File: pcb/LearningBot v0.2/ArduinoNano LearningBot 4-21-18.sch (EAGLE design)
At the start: 22 parts

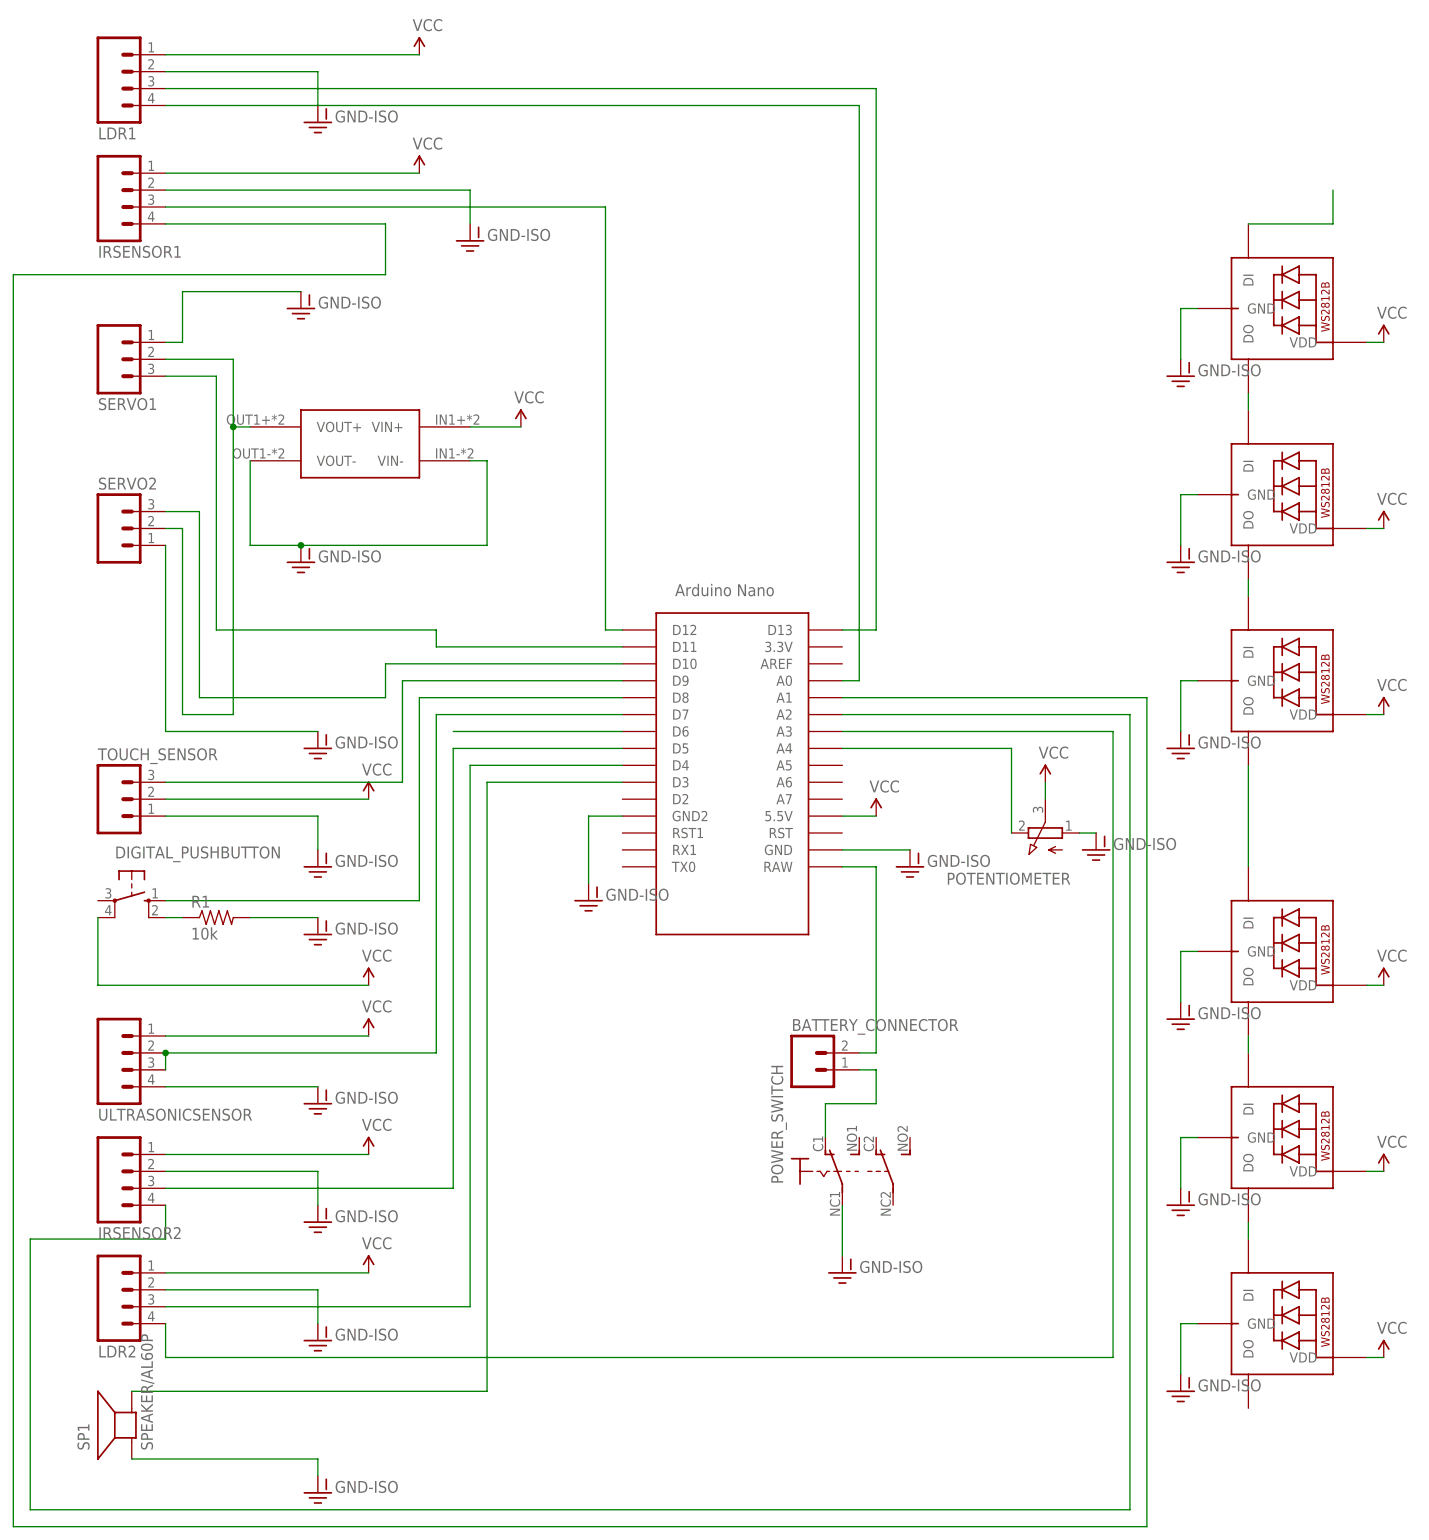
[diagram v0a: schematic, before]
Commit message: Ready for inspection
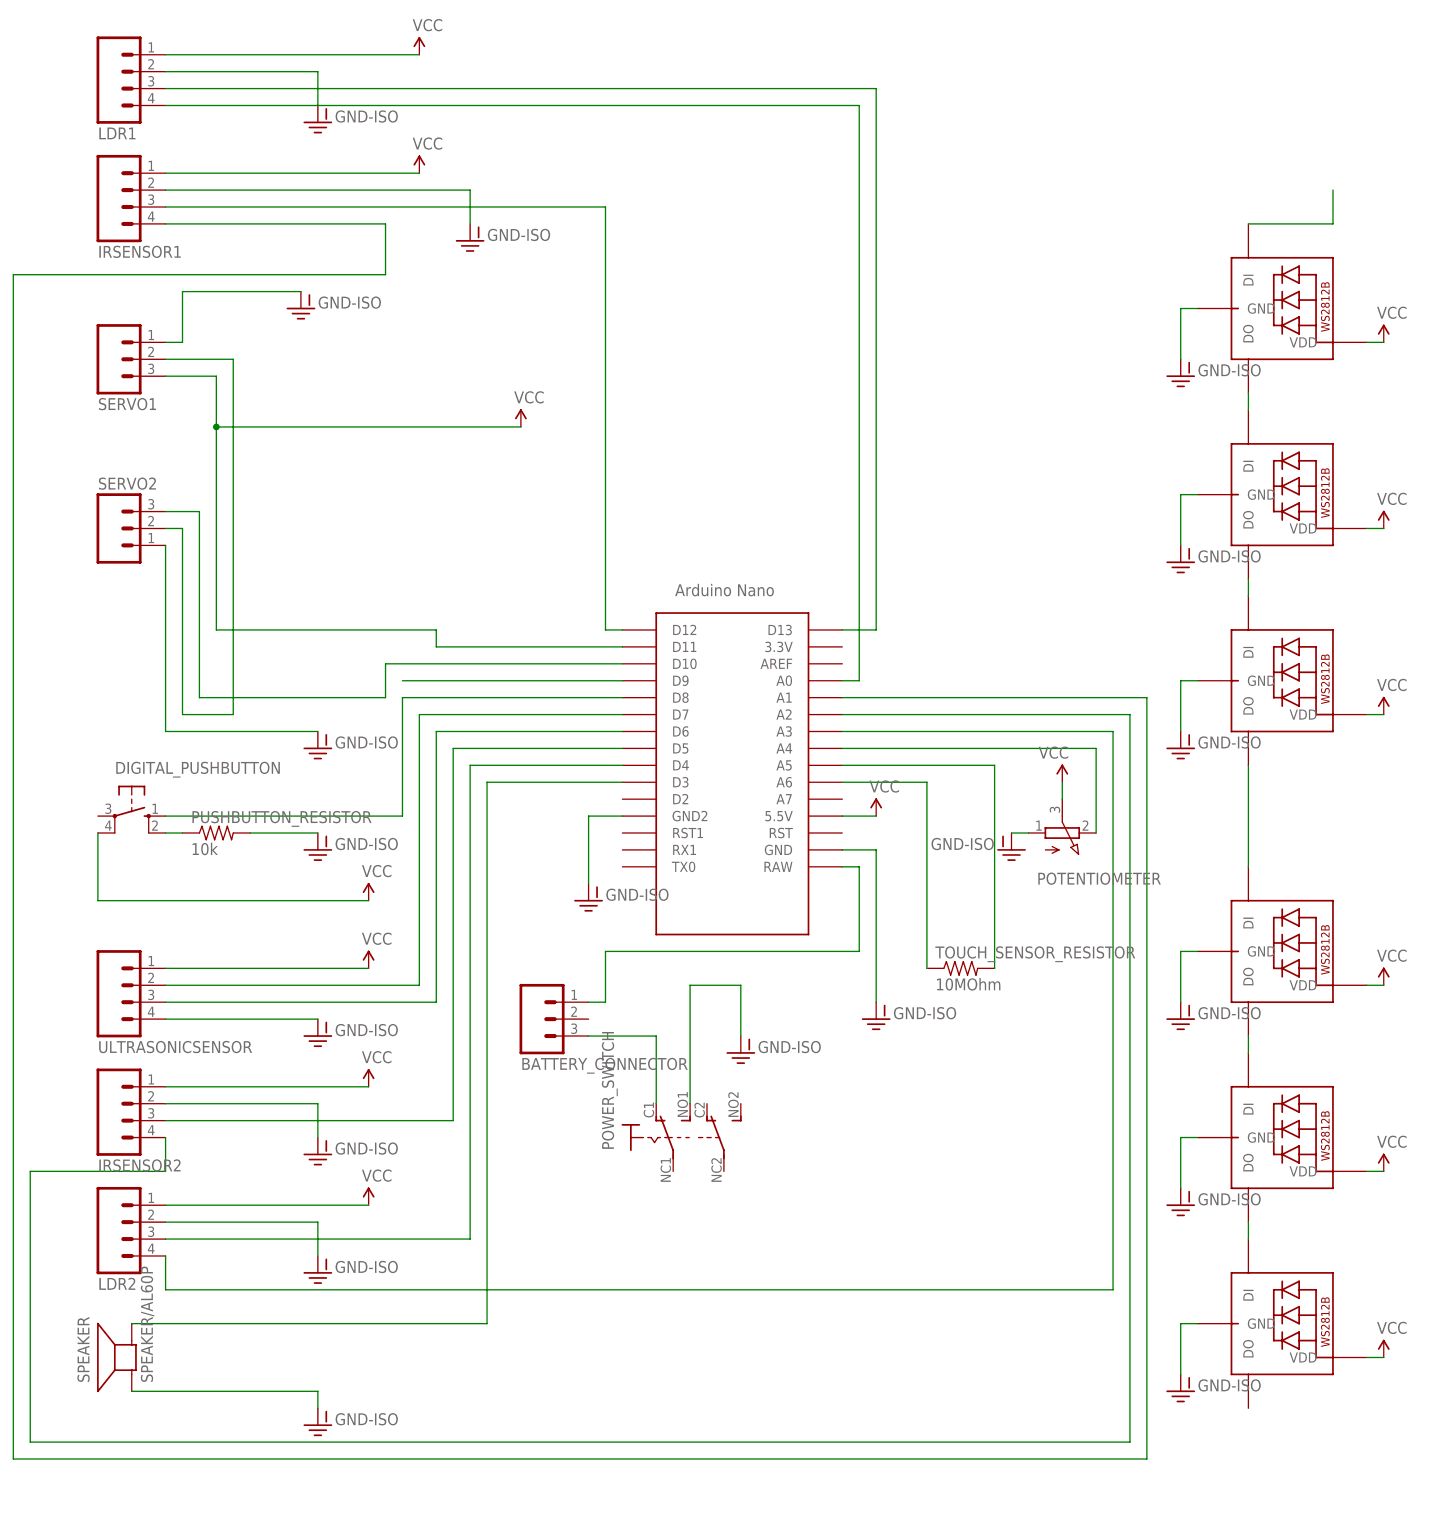
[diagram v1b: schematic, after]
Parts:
- removed R1: 10k, SparkFun-Passives:RESISTORPTH-1/4W
- removed SP1: SPEAKER/AL60P, adafruit:SPEAKER/AL60P
- removed TOUCH_SENSOR: (no value), SparkFun-Connectors:M03LOCK
- removed U$3: MP1584, MP1584-dc-brick:MP1584
- added PUSHBUTTON_RESISTOR: 10k, SparkFun-Passives:RESISTORPTH-1/4W
- added SPEAKER: SPEAKER/AL60P, adafruit:SPEAKER/AL60P
- added TOUCH_SENSOR_RESISTOR: 10MOhm, SparkFun-Passives:RESISTORPTH-1/4W
- BATTERY_CONNECTOR: device SparkFun-Connectors:M02-JST-2-PTH-NO_SILK -> SparkFun-Connectors:M03JST-PTH-VERT
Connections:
- removed net SERVO1_PIN: SERVO1.3, U$1.D11
- removed net TOUCH_SENSOR: TOUCH_SENSOR.3, U$1.D9
- removed net ULTRASONICSENSOR_PIN: U$1.D7, ULTRASONICSENSOR.2, ULTRASONICSENSOR.3
- new net CAP_TOUCH_RECEIVE_PIN: TOUCH_SENSOR_RESISTOR.1, U$1.A6
- new net CAP_TOUCH_SEND_PIN: TOUCH_SENSOR_RESISTOR.2, U$1.A5
- new net ECHO_PIN: U$1.D6, ULTRASONICSENSOR.3
- new net TRIG_PIN: U$1.D7, ULTRASONICSENSOR.2
- net GND: now also POWER_SWITCH1.S, PUSHBUTTON_RESISTOR.2, SPEAKER.+; no longer POWER_SWITCH1.P, R1.2, SP1.+, TOUCH_SENSOR.1, U$3.VIN-, U$3.VOUT-
- net LED-1: now also U$1.D9; no longer U$1.D6
- net N$3: now also PUSHBUTTON_RESISTOR.1; no longer R1.1
- net N$9: now also BATTERY_CONNECTOR.3; no longer BATTERY_CONNECTOR.1
- net RAWIN: now also BATTERY_CONNECTOR.1; no longer BATTERY_CONNECTOR.2
- net SERVOVCC: no longer U$3.VOUT+
- net SPEAKERPIN: now also SPEAKER.-; no longer SP1.-
- net VCC: now also SERVO1.3, U$1.D11; no longer TOUCH_SENSOR.2, U$3.VIN+
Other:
- moved on the sheet: DIGITAL_PUSHBUTTON, IRSENSOR2, LDR2, POTENTIOMETER, POWER_SWITCH, ULTRASONICSENSOR
